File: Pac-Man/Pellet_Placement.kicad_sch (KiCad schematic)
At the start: 9 parts, among them U23 74LS74, U24 74LS74, U25 74LS74, U26 27C64, U27 74LS74, U28 74LS74, U29 74LS74, U30 74LS74, U31 ICM7555xB

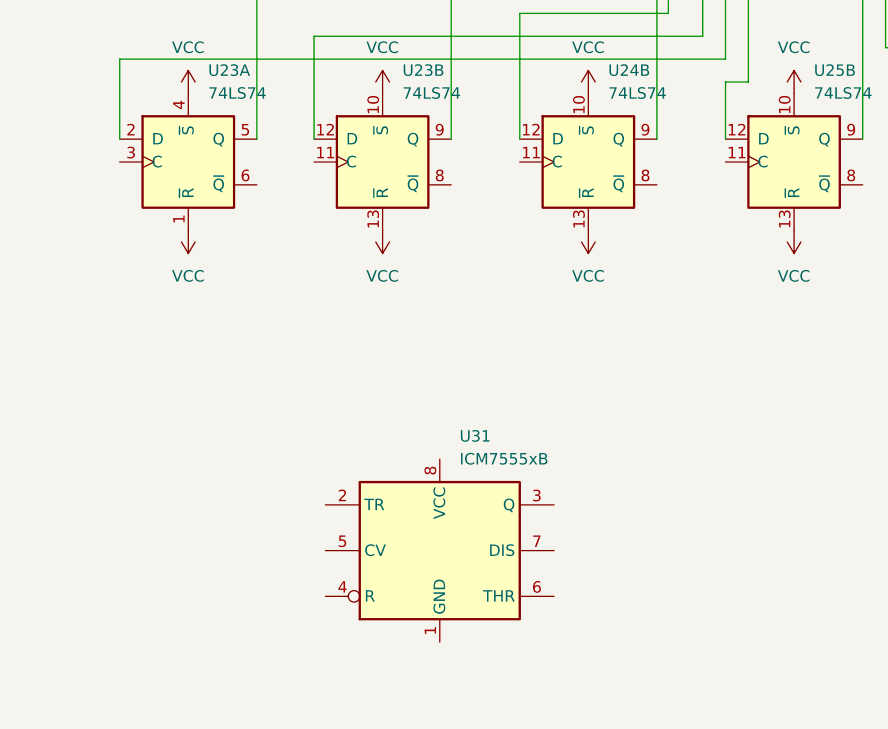
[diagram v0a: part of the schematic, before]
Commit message: Add files via upload
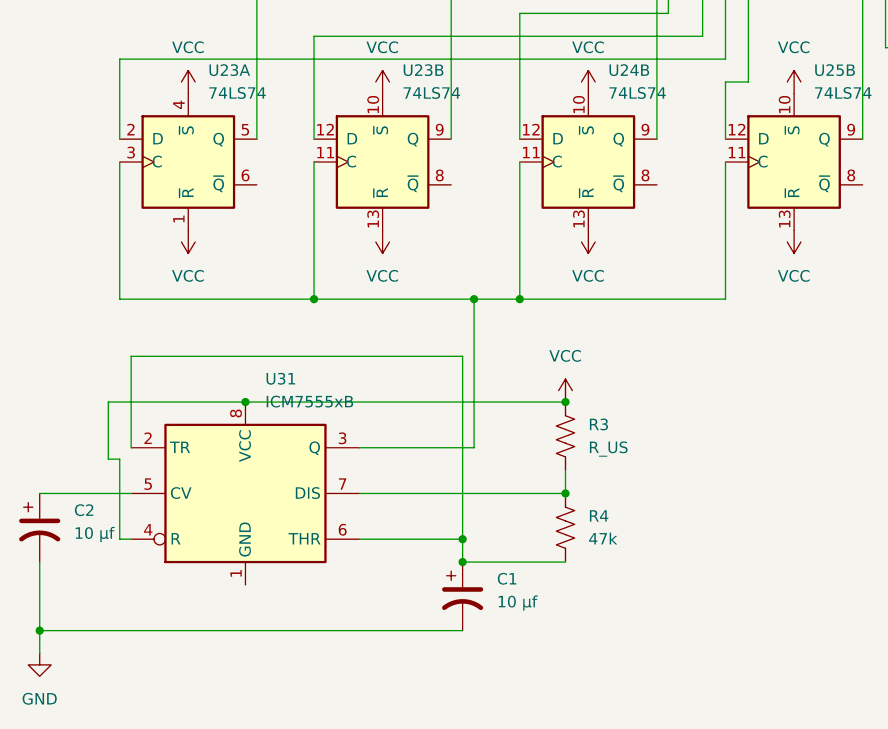
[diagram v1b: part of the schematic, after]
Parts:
- added C1, C2: 10 μf, symbol Device:C_Polarized_US
- added R3: R_US, symbol Device:R_US
- added R4: 47k, symbol Device:R_US
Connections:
- net GND: now also C1.2, C2.2
- net VCC: now also U31.4 (R), U31.8 (VCC), R3.1
- net at U24.11 (C): now also U23.11 (C), U23.3 (C), U25.11 (C), U31.3 (Q)
- net at U31.2 (TR): now also U31.6 (THR), C1.1, R4.2
- net at U31.5 (CV): now also C2.1
- net at U31.7 (DIS): now also R3.2, R4.1
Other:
- moved on the sheet: U31
